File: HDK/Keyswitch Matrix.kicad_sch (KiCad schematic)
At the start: 166 parts

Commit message: updated pcb
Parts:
- D201, D202, D203, D204, D205, D206, D207, D208, D209, D210, D211, D212, D213, D214, D215, D216, D217, D218, D219, D220, D221, D222, D223, D224, D225, D226, D227, D228, D229, D230, D231, D232, D233, D234, D235, D236, D237, D238, D239, D240, D241, D242, D243, D244, D245, D246, D247, D248, D249, D250, D251, D252, D253, D254, D255, D256, D257, D258, D259, D260, D261, D262, D263, D264, D265, D266, D267, D268, D269, D270, D271, D272, D273, D274, D275, D276, D277, D278, D279, D280, D281, D282, D283: symbol Device:D -> x83-kb-lib:D
- SW201, SW202, SW203, SW204, SW205, SW206, SW207, SW208, SW209, SW210, SW211, SW212, SW213, SW214, SW215, SW216, SW217, SW218, SW219, SW220, SW221, SW222, SW223, SW224, SW225, SW226, SW227, SW228, SW229, SW230, SW232, SW233, SW234, SW235, SW236, SW237, SW238, SW239, SW240, SW241, SW242, SW243, SW244, SW245, SW247, SW248, SW249, SW250, SW251, SW252, SW253, SW254, SW255, SW256, SW257, SW258, SW259, SW261, SW262, SW263, SW264, SW265, SW266, SW267, SW268, SW269, SW270, SW271, SW272, SW273, SW274, SW275, SW276, SW277, SW278, SW279, SW280, SW281, SW282, SW283: footprint sckb-footprint:Optional Hotswap MX 1.00U -> x83-kb-lib:SW_OPT_MX; symbol sckb-parts:HS/S-keyswitch -> x83-kb-lib:HS/S-keyswitch
- SW231, SW246, SW260: footprint sckb-footprint:Optional Hotswap MX 1.00U -> x83-kb-lib:SW_OPT_MX; symbol sckb-parts:S-Keyswitch/ Rotary Encoder -> x83-kb-lib:S-Keyswitch/ Rotary Encoder
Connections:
- net at SW253.1 (A): now also SW252.1 (A); no longer SW254.1 (A)
- net at SW252.1 (A): now also SW251.1 (A); no longer SW253.1 (A)
- net at SW262.1 (A): now also SW261.1 (A); no longer SW263.1 (A)
- net at SW220.1 (A): now also SW221.1 (A); no longer SW219.1 (A)
- net at SW221.1 (A): now also SW222.1 (A); no longer SW220.1 (A)
- net at SW248.1 (A): now also SW249.1 (A); no longer SW247.1 (A)
- net at SW249.1 (A): now also SW250.1 (A); no longer SW248.1 (A)
- net at SW240.1 (A): now also SW241.1 (A); no longer SW239.1 (A)
- net at SW241.1 (A): now also SW242.1 (A); no longer SW240.1 (A)
- net at SW209.1 (A): now also SW208.1 (A); no longer SW210.1 (A)
- net at SW208.1 (A): now also SW207.1 (A); no longer SW209.1 (A)
- net at SW276.1 (A): now also SW275.1 (A); no longer SW277.1 (A)
- net at SW275.1 (A): now also SW274.1 (A); no longer SW276.1 (A)
- net at SW230.1 (A): now also SW231.1 (A); no longer SW229.1 (A)
- net at SW233.1 (A): now also SW232.1 (A); no longer SW234.1 (A)
- net at SW244.1 (A): now also SW245.1 (A); no longer SW243.1 (A)
- net at SW245.1 (A): now also SW246.1 (A); no longer SW244.1 (A)
- net at SW204.1 (A): now also SW205.1 (A); no longer SW203.1 (A)
- net at SW205.1 (A): now also SW206.1 (A); no longer SW204.1 (A)
- net at SW273.1 (A): now also SW272.1 (A)
- net at SW272.1 (A): now also SW271.1 (A); no longer SW273.1 (A)
- net at SW214.1 (A): now also SW215.1 (A); no longer SW213.1 (A)
- net at SW215.1 (A): now also SW216.1 (A); no longer SW214.1 (A)
- net at SW257.1 (A): now also SW258.1 (A); no longer SW256.1 (A)
- net at SW216.1 (A): no longer SW215.1 (A)
- net at SW250.1 (A): now also SW251.1 (A); no longer SW249.1 (A)
- net at SW228.1 (A): now also SW229.1 (A); no longer SW227.1 (A)
- net at SW283.1 (A): now also SW282.1 (A)
- net at SW282.1 (A): now also SW281.1 (A); no longer SW283.1 (A)
- net at SW206.1 (A): now also SW207.1 (A); no longer SW205.1 (A)
- net at SW269.1 (A): now also SW268.1 (A); no longer SW270.1 (A)
- net at SW268.1 (A): now also SW267.1 (A); no longer SW269.1 (A)
- net at SW218.1 (A): now also SW219.1 (A); no longer SW217.1 (A)
- net at SW281.1 (A): now also SW280.1 (A); no longer SW282.1 (A)
- net at SW222.1 (A): now also SW223.1 (A); no longer SW221.1 (A)
- new net: SW253.1 (A), SW254.1 (A)
- new net: SW262.1 (A), SW263.1 (A)
- new net: SW219.1 (A), SW220.1 (A)
- new net: SW247.1 (A), SW248.1 (A)
- new net: SW239.1 (A), SW240.1 (A)
- new net: SW209.1 (A), SW210.1 (A)
- new net: SW276.1 (A), SW277.1 (A)
- new net: SW229.1 (A), SW230.1 (A)
- new net: SW233.1 (A), SW234.1 (A)
- new net: SW243.1 (A), SW244.1 (A)
- new net: SW203.1 (A), SW204.1 (A)
- new net: SW213.1 (A), SW214.1 (A)
- new net: SW256.1 (A), SW257.1 (A)
- new net: SW227.1 (A), SW228.1 (A)
- new net: SW269.1 (A), SW270.1 (A)
- new net: SW217.1 (A), SW218.1 (A)

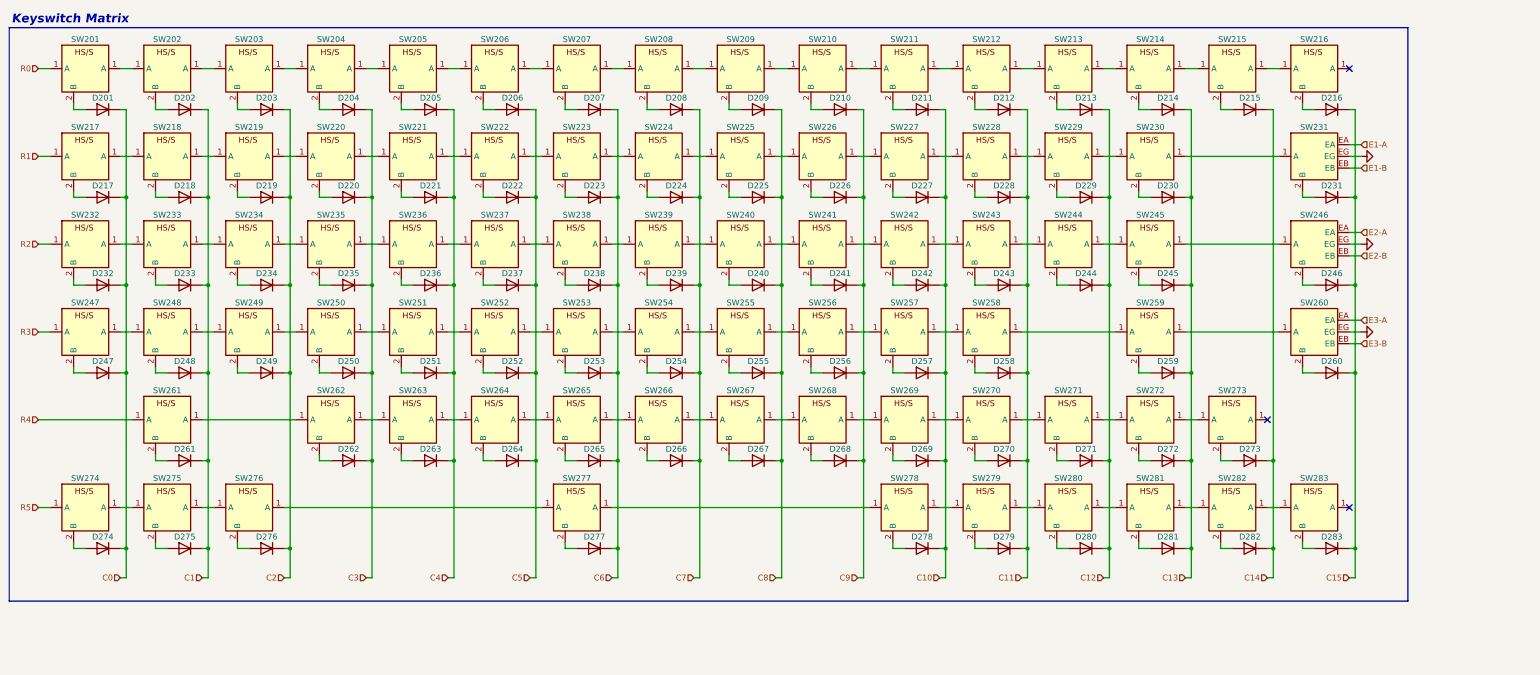
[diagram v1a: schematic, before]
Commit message: updated pcb
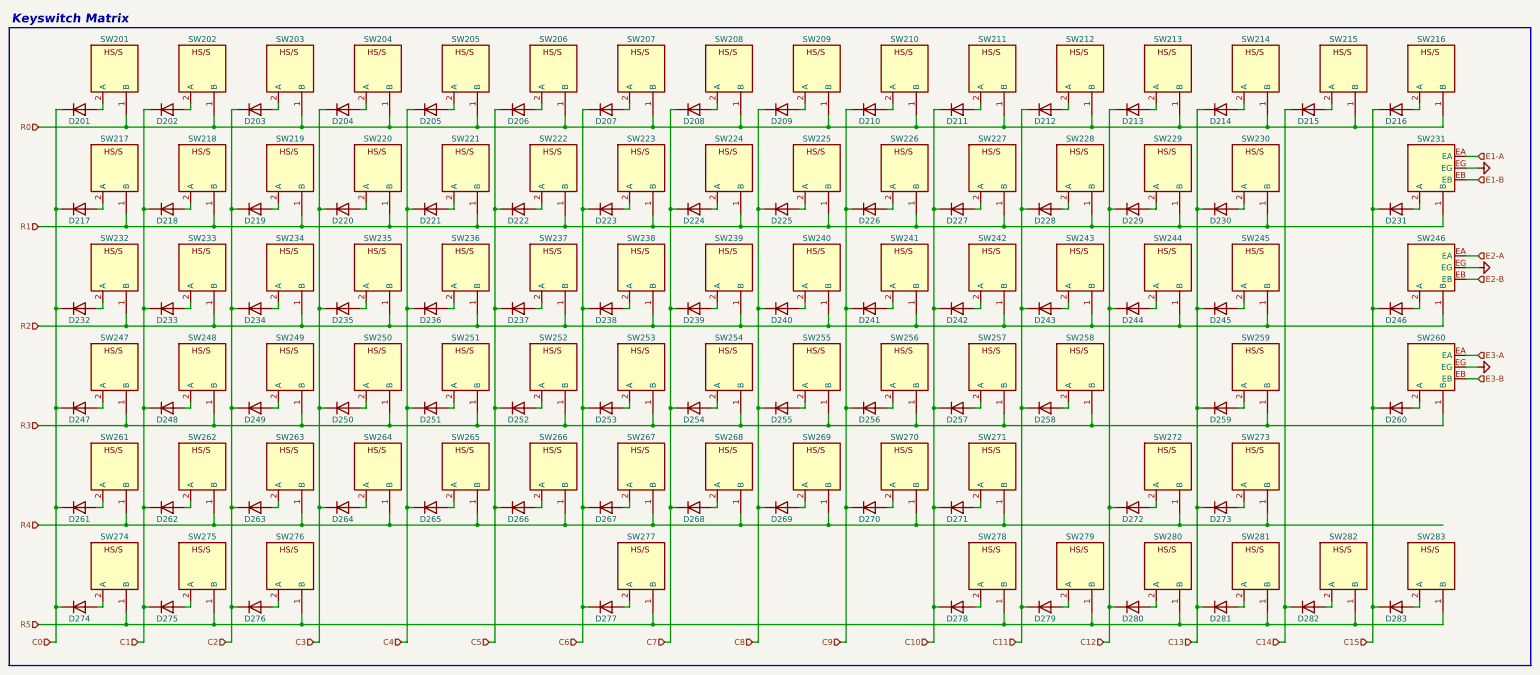
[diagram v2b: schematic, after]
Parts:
- removed SW201, SW202, SW203, SW204, SW205, SW206, SW207, SW208, SW209, SW210, SW211, SW212, SW213, SW214, SW215, SW216, SW217, SW218, SW219, SW220, SW221, SW222, SW223, SW224, SW225, SW226, SW227, SW228, SW229, SW230, SW232, SW233, SW234, SW235, SW236, SW237, SW238, SW239, SW240, SW241, SW242, SW243, SW244, SW245, SW247, SW248, SW249, SW250, SW251, SW252, SW253, SW254, SW255, SW256, SW257, SW258, SW259, SW261, SW262, SW263, SW264, SW265, SW266, SW267, SW268, SW269, SW270, SW271, SW272, SW273, SW274, SW275, SW276, SW277, SW278, SW279, SW280, SW281, SW282, SW283: ~, x83-kb-lib:SW_OPT_MX, symbol x83-kb-lib:HS/S-keyswitch
- added SW201, SW202, SW203, SW204, SW205, SW206, SW207, SW208, SW209, SW210, SW211, SW212, SW213, SW214, SW215, SW216, SW217, SW218, SW219, SW220, SW221, SW222, SW223, SW224, SW225, SW226, SW227, SW228, SW229, SW230, SW232, SW233, SW234, SW235, SW236, SW237, SW238, SW239, SW240, SW241, SW242, SW243, SW244, SW245, SW247, SW248, SW249, SW250, SW251, SW252, SW253, SW254, SW255, SW256, SW257, SW258, SW259, SW261, SW262, SW263, SW264, SW265, SW266, SW267, SW268, SW269, SW270, SW271, SW272, SW273, SW274, SW275, SW276, SW277, SW278, SW279, SW280, SW281, SW282, SW283: ~, x83-kb-lib:SW_OPT_MX, symbol x83-kb-lib:HS/S-keyswitch_1
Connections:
- net C0: now also D261.1 (K)
- net C1: now also D262.1 (K); no longer D261.1 (K)
- net C10: now also D271.1 (K); no longer D269.1 (K)
- net C11: no longer D270.1 (K)
- net C12: now also D272.1 (K); no longer D271.1 (K)
- net C13: now also D273.1 (K); no longer D272.1 (K)
- net C14: no longer D273.1 (K)
- net C2: now also D263.1 (K)
- net C3: now also D264.1 (K); no longer D262.1 (K)
- net C4: now also D265.1 (K); no longer D263.1 (K)
- net C5: now also D266.1 (K); no longer D264.1 (K)
- net C6: now also D267.1 (K); no longer D265.1 (K)
- net C7: now also D268.1 (K); no longer D266.1 (K)
- net C8: now also D269.1 (K); no longer D267.1 (K)
- net C9: now also D270.1 (K); no longer D268.1 (K)
- net R0: now also SW201.1 (B), SW202.1 (B), SW203.1 (B), SW204.1 (B), SW205.1 (B), SW206.1 (B), SW207.1 (B), SW208.1 (B), SW209.1 (B), SW210.1 (B), SW211.1 (B), SW212.1 (B), SW213.1 (B), SW214.1 (B), SW215.1 (B), SW216.1 (B)
- net R1: now also SW231.1 (B), SW217.1 (B), SW218.1 (B), SW219.1 (B), SW220.1 (B), SW221.1 (B), SW222.1 (B), SW223.1 (B), SW224.1 (B), SW225.1 (B), SW226.1 (B), SW227.1 (B), SW228.1 (B), SW229.1 (B), SW230.1 (B)
- net R2: now also SW246.1 (B), SW232.1 (B), SW233.1 (B), SW234.1 (B), SW235.1 (B), SW236.1 (B), SW237.1 (B), SW238.1 (B), SW239.1 (B), SW240.1 (B), SW241.1 (B), SW242.1 (B), SW243.1 (B), SW244.1 (B), SW245.1 (B)
- net R3: now also SW260.1 (B), SW247.1 (B), SW248.1 (B), SW249.1 (B), SW250.1 (B), SW251.1 (B), SW252.1 (B), SW253.1 (B), SW254.1 (B), SW255.1 (B), SW256.1 (B), SW257.1 (B), SW258.1 (B), SW259.1 (B)
- net R4: now also SW261.1 (B), SW262.1 (B), SW263.1 (B), SW264.1 (B), SW265.1 (B), SW266.1 (B), SW267.1 (B), SW268.1 (B), SW269.1 (B), SW270.1 (B), SW271.1 (B), SW272.1 (B), SW273.1 (B)
- net R5: now also SW274.1 (B), SW275.1 (B), SW276.1 (B), SW277.1 (B), SW278.1 (B), SW279.1 (B), SW280.1 (B), SW281.1 (B), SW282.1 (B), SW283.1 (B)
- net at D253.2 (A): now also SW253.2 (A)
- net at D262.2 (A): now also SW262.2 (A)
- net at D279.2 (A): now also SW279.2 (A)
- net at D220.2 (A): now also SW220.2 (A)
- net at D258.2 (A): now also SW258.2 (A)
- net at D265.2 (A): now also SW265.2 (A)
- net at D214.2 (A): now also SW214.2 (A)
- net at D225.2 (A): now also SW225.2 (A)
- net at D248.2 (A): now also SW248.2 (A)
- net at D259.2 (A): now also SW259.2 (A)
- net at D263.2 (A): now also SW263.2 (A)
- net at D240.2 (A): now also SW240.2 (A)
- net at D238.2 (A): now also SW238.2 (A)
- net at D209.2 (A): now also SW209.2 (A)
- net at D283.2 (A): now also SW283.2 (A)
- net at D219.2 (A): now also SW219.2 (A)
- net at D276.2 (A): now also SW276.2 (A)
- net at D230.2 (A): now also SW230.2 (A)
- net at D261.2 (A): now also SW261.2 (A)
- net at D233.2 (A): now also SW233.2 (A)
- net at D223.2 (A): now also SW223.2 (A)
- net at D242.2 (A): now also SW242.2 (A)
- net at D213.2 (A): now also SW213.2 (A)
- net at D210.2 (A): now also SW210.2 (A)
- net at D215.2 (A): now also SW215.2 (A)
- net at D244.2 (A): now also SW244.2 (A)
- net at D271.2 (A): now also SW271.2 (A)
- net at D229.2 (A): now also SW229.2 (A)
- net at D239.2 (A): now also SW239.2 (A)
- net at D228.2 (A): now also SW228.2 (A)
- net at D268.2 (A): now also SW268.2 (A)
- net at D277.2 (A): now also SW277.2 (A)
- net at D204.2 (A): now also SW204.2 (A)
- net at D250.2 (A): now also SW250.2 (A)
- net at D227.2 (A): now also SW227.2 (A)
- net at D249.2 (A): now also SW249.2 (A)
- net at D243.2 (A): now also SW243.2 (A)
- net at D273.2 (A): now also SW273.2 (A)
- net at D235.2 (A): now also SW235.2 (A)
- net at D272.2 (A): now also SW272.2 (A)
- net at D270.2 (A): now also SW270.2 (A)
- net at D234.2 (A): now also SW234.2 (A)
- net at D203.2 (A): now also SW203.2 (A)
- net at D278.2 (A): now also SW278.2 (A)
- net at D221.2 (A): now also SW221.2 (A)
- net at D202.2 (A): now also SW202.2 (A)
- net at D232.2 (A): now also SW232.2 (A)
- net at D254.2 (A): now also SW254.2 (A)
- net at D274.2 (A): now also SW274.2 (A)
- net at D257.2 (A): now also SW257.2 (A)
- net at D236.2 (A): now also SW236.2 (A)
- net at D212.2 (A): now also SW212.2 (A)
- net at D255.2 (A): now also SW255.2 (A)
- net at D205.2 (A): now also SW205.2 (A)
- net at D201.2 (A): now also SW201.2 (A)
- net at D251.2 (A): now also SW251.2 (A)
- net at D280.2 (A): now also SW280.2 (A)
- net at D217.2 (A): now also SW217.2 (A)
- net at D206.2 (A): now also SW206.2 (A)
- net at D216.2 (A): now also SW216.2 (A)
- net at D207.2 (A): now also SW207.2 (A)
- net at D264.2 (A): now also SW264.2 (A)
- net at D252.2 (A): now also SW252.2 (A)
- net at D241.2 (A): now also SW241.2 (A)
- net at D226.2 (A): now also SW226.2 (A)
- net at D269.2 (A): now also SW269.2 (A)
- net at D211.2 (A): now also SW211.2 (A)
- net at D247.2 (A): now also SW247.2 (A)
- net at D256.2 (A): now also SW256.2 (A)
- net at D245.2 (A): now also SW245.2 (A)
- net at D266.2 (A): now also SW266.2 (A)
- net at D218.2 (A): now also SW218.2 (A)
- net at D282.2 (A): now also SW282.2 (A)
- net at D224.2 (A): now also SW224.2 (A)
- net at D208.2 (A): now also SW208.2 (A)
- net at D267.2 (A): now also SW267.2 (A)
- net at D275.2 (A): now also SW275.2 (A)
- net at D281.2 (A): now also SW281.2 (A)
- net at D237.2 (A): now also SW237.2 (A)
- net at D222.2 (A): now also SW222.2 (A)
- no-connect marks 3 -> 0

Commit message: added models
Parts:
- SW201, SW202, SW203, SW204, SW205, SW206, SW207, SW208, SW209, SW210, SW211, SW212, SW213, SW214, SW215, SW216, SW217, SW218, SW219, SW220, SW221, SW222, SW223, SW224, SW225, SW226, SW227, SW228, SW229, SW230, SW232, SW233, SW234, SW235, SW236, SW237, SW238, SW239, SW240, SW241, SW242, SW243, SW244, SW245, SW247, SW248, SW249, SW250, SW251, SW252, SW253, SW254, SW255, SW256, SW257, SW258, SW259, SW261, SW262, SW263, SW264, SW265, SW266, SW267, SW268, SW269, SW270, SW271, SW272, SW273, SW274, SW275, SW276, SW277, SW278, SW279, SW280, SW281, SW282, SW283: symbol x83-kb-lib:HS/S-keyswitch_1 -> x83-kb-lib:Keyswitch
